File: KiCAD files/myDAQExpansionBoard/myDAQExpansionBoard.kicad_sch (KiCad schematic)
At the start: 48 parts, among them J1 OSTV7XX3151

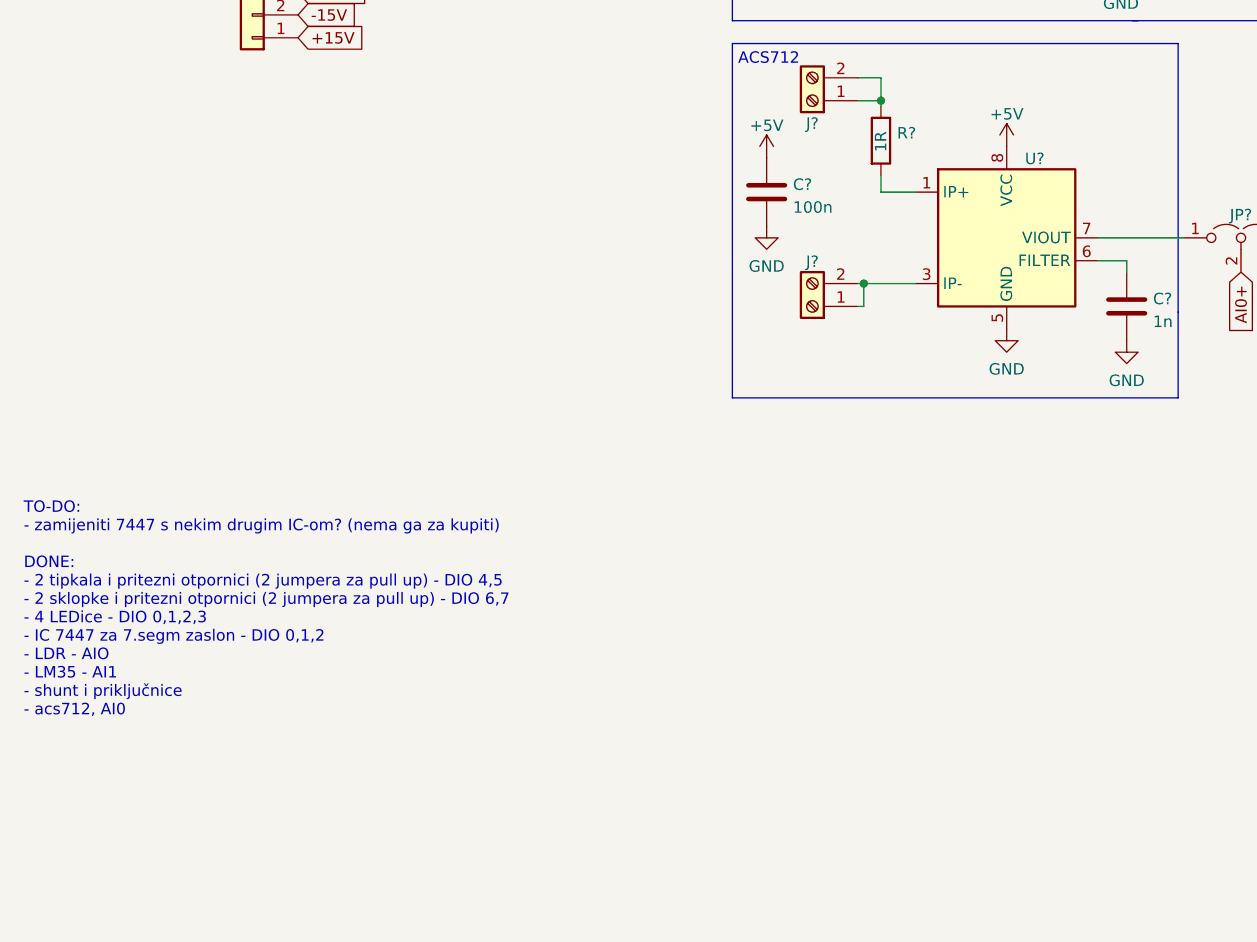
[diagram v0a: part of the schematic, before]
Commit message: update
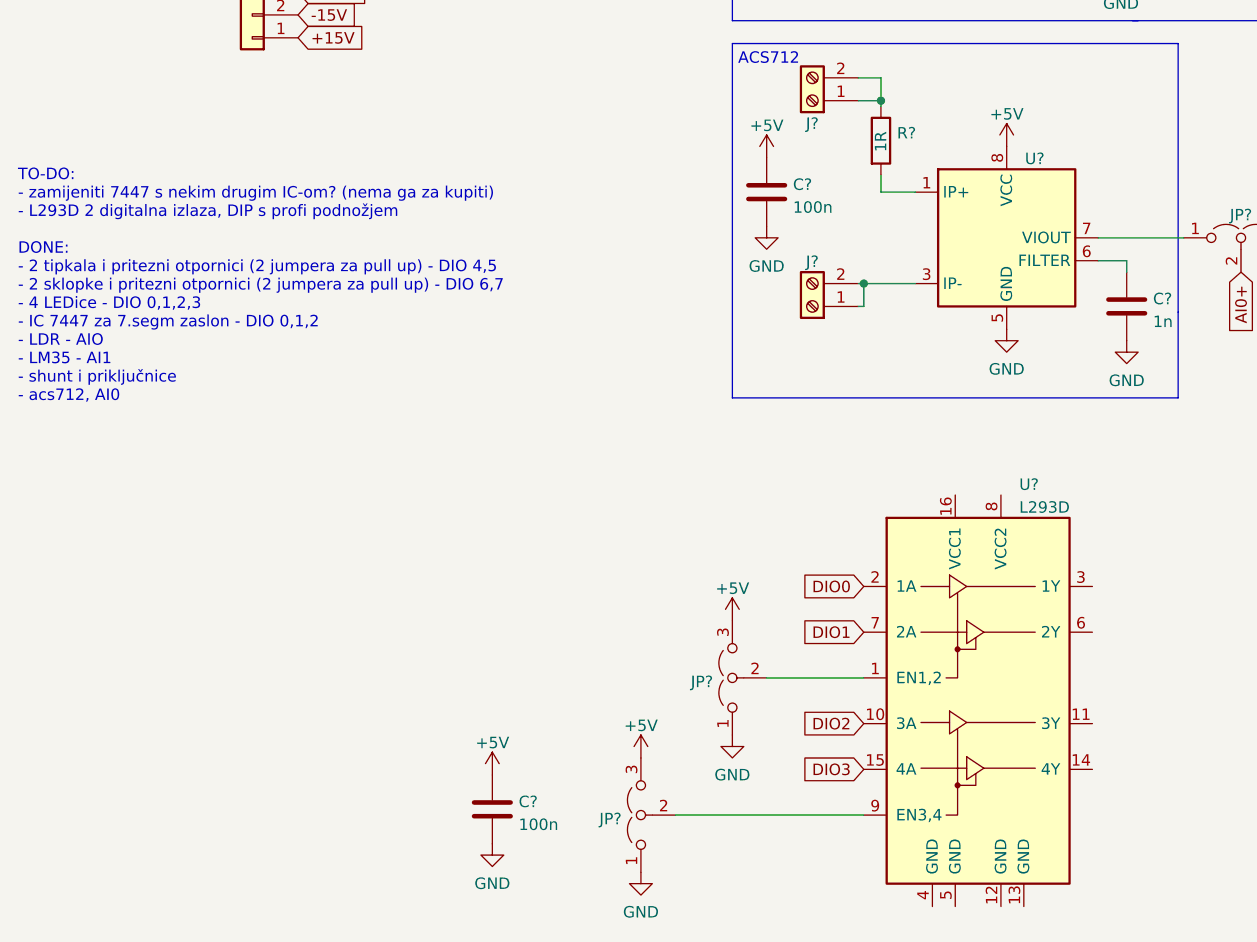
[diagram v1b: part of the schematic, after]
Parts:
- added C?: 100n, symbol Device:C
- added JP? (x2): Jumper_3_Open, symbol Jumper:Jumper_3_Open
- added U?: L293D, Package_DIP:DIP-16_W7.62mm, symbol Driver_Motor:L293D
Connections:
- net +5V: now also C?.1, JP?.3 (B), JP?.3 (B)
- net DIO0: now also U?.2 (1A)
- net DIO1: now also U?.7 (2A)
- net DIO2: now also U?.10 (3A)
- net DIO3: now also U?.15 (4A)
- net GND: now also C?.2, JP?.1 (A), JP?.1 (A)
- new net: JP?.2 (C), U?.1 (EN1,2)
- new net: JP?.2 (C), U?.9 (EN3,4)
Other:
- note added: "TO-DO: - zamijeniti 7447 s nekim drugim IC-om? (nema ga za kupiti) - L293D 2 digitalna izlaza, DIP s profi podnožjem DONE: - 2 tipkala i pritezni otpornici (2 jumpera za pull up) - DIO 4,5 - 2 sklopke i pritezni otpornici (2 jumpera za pull up) - DIO 6,7 - 4 LEDice - DIO 0,1,2,3 - IC 7447 za 7.segm zaslon - DIO 0,1,2 - LDR - AIO - LM35 - AI1 - shunt i priključnice - acs712, AI0"
- note removed: "TO-DO: - zamijeniti 7447 s nekim drugim IC-om? (nema ga za kupiti) DONE: - 2 tipkala i pritezni otpornici (2 jumpera za pull up) - DIO 4,5 - 2 sklopke i pritezni otpornici (2 jumpera za pull up) - DIO 6,7 - 4 LEDice - DIO 0,1,2,3 - IC 7447 za 7.segm zaslon - DIO 0,1,2 - LDR - AIO - LM35 - AI1 - shunt i priključnice - acs712, AI0"

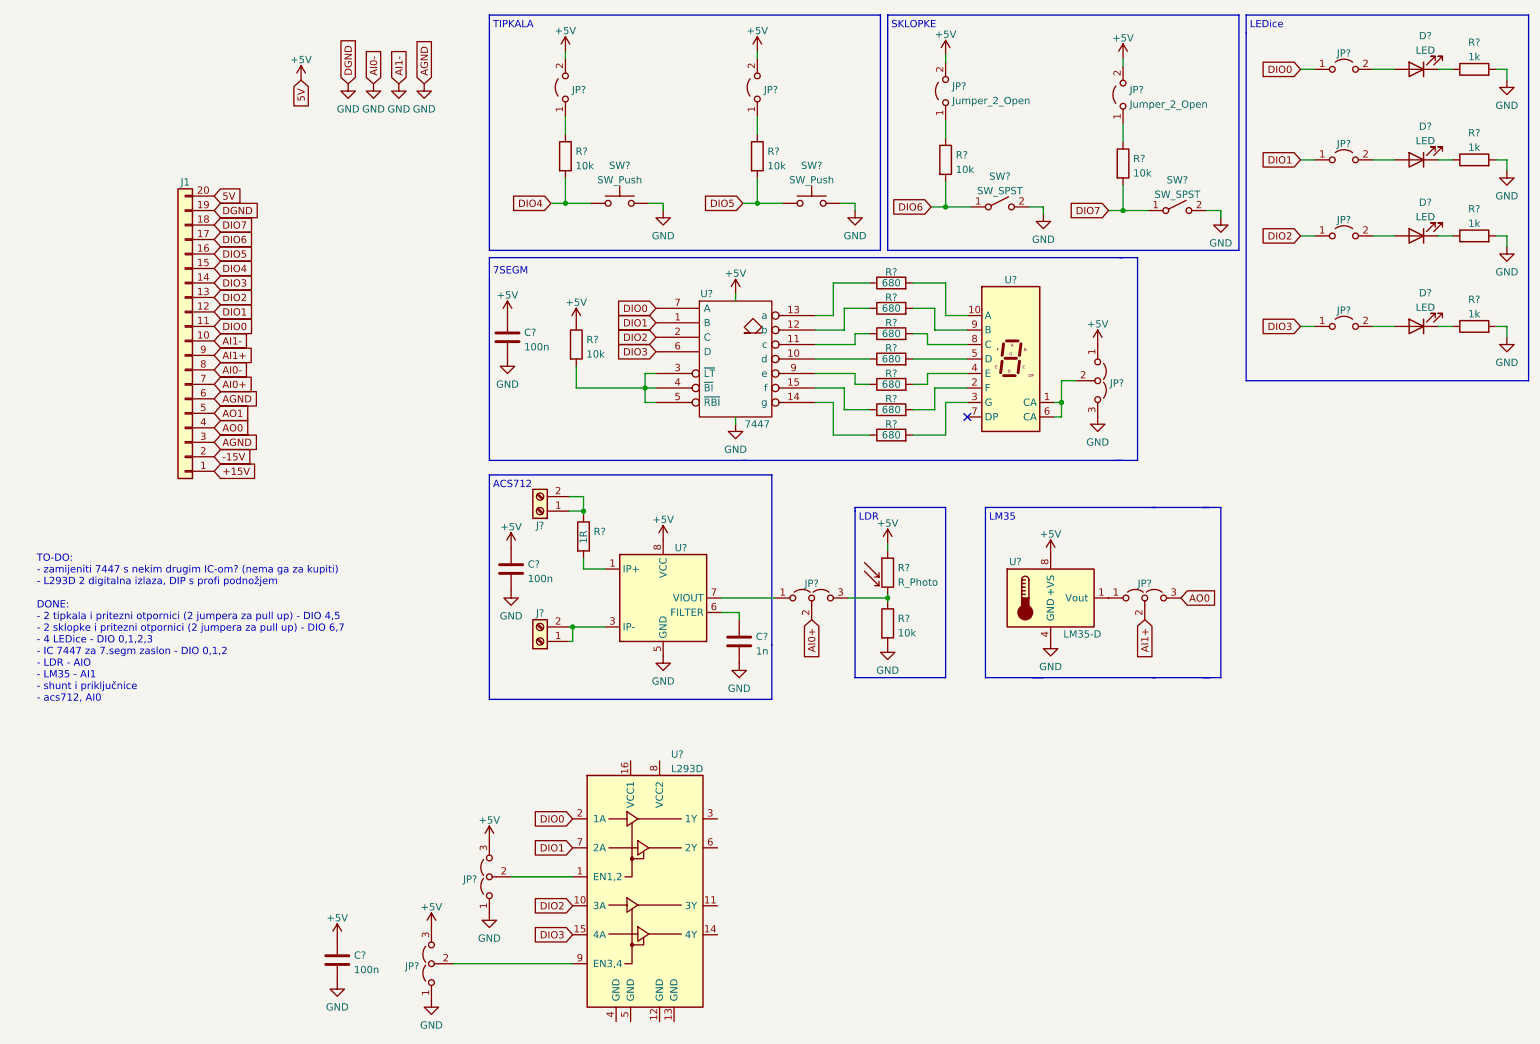
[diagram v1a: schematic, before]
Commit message: Update myDAQExpansionBoard.kicad_sch
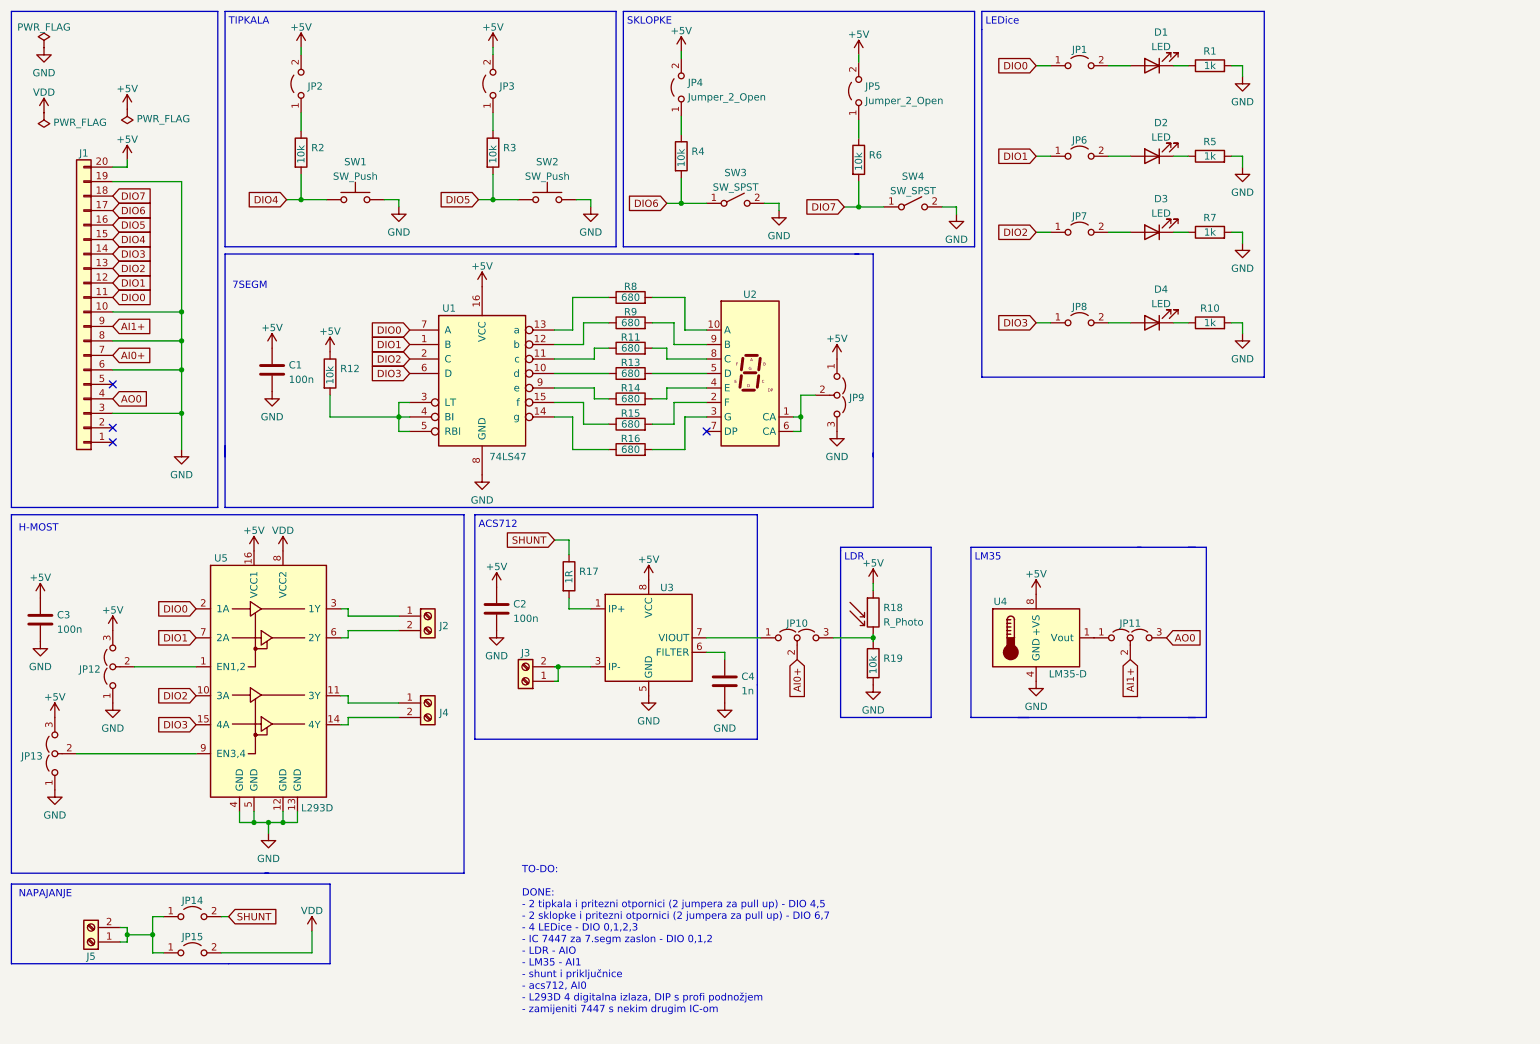
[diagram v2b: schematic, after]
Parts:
- removed U?: 7447, symbol 74xx_IEEE:7447
- added J2, J4: Screw_Terminal_01x02, symbol Connector:Screw_Terminal_01x02
- added JP14, JP15: Jumper_2_Open, symbol Jumper:Jumper_2_Open
- added U1: 74LS47, Package_DIP:DIP-16_W7.62mm, symbol 74xx:74LS47
- D1, D2, D3, D4: renamed from D?; footprint (none) -> LED_THT:LED_D5.0mm
- J1: footprint (none) -> Library:OSTV7XX3151
- gave numbers to parts that had none: 46
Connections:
- net +5V: now also U5.16 (VCC1), U1.16 (VCC)
- net DIO0: now also U1.7 (A)
- net DIO1: now also U1.1 (B)
- net DIO2: now also U1.2 (C)
- net DIO3: now also U1.6 (D)
- net GND: now also U5.12 (GND), U5.13 (GND), U5.4 (GND), U5.5 (GND), U1.8 (GND)
- net at U5.11 (3Y): now also J4.1 (Pin_1)
- net at U5.14 (4Y): now also J4.2 (Pin_2)
- net at U5.3 (1Y): now also J2.1 (Pin_1)
- net at U5.6 (2Y): now also J2.2 (Pin_2)
- net VDD: now reaches U5.8 (VCC2)
- net VDD: now also JP15.2 (B)
- net at R8.1: now also U1.13 (a)
- net at R9.1: now also U1.12 (b)
- net at R13.1: now also U1.10 (d)
- net at R11.1: now also U1.11 (c)
- net at R16.1: now also U1.14 (g)
- net at R15.1: now also U1.15 (f)
- net at R12.2: now also U1.3 (LT), U1.4 (BI), U1.5 (RBI)
- net at R14.1: now also U1.9 (e)
- net at J5.1 (Pin_1), J5.2 (Pin_2): now also JP14.1 (A), JP15.1 (A); no longer R17.1
- net +15V: no longer names the net of J1.1 (Pin_1)
- net -15V: no longer names the net of J1.2 (Pin_2)
- net AO1: no longer names the net of J1.5 (Pin_5)
- new net SHUNT: JP14.2 (B), R17.1
- no-connect marks 1 -> 4
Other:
- note added: "H-MOST"
- note added: "NAPAJANJE"
- note added: "TO-DO: DONE: - 2 tipkala i pritezni otpornici (2 jumpera za pull up) - DIO 4,5 - 2 sklopke i pritezni otpornici (2 jumpera za pull up) - DIO 6,7 - 4 LEDice - DIO 0,1,2,3 - IC 7447 za 7.segm zaslon - DIO 0,1,2 - LDR - AIO - LM35 - AI1 - shunt i priključnice - acs712, AI0 - L293D 4 digitalna izlaza, DIP s profi podnožjem - zamijeniti 7447 s nekim drugim IC-om"
- note removed: "TO-DO: - zamijeniti 7447 s nekim drugim IC-om? (nema ga za kupiti) - L293D 2 digitalna izlaza, DIP s profi podnožjem DONE: - 2 tipkala i pritezni otpornici (2 jumpera za pull up) - DIO 4,5 - 2 sklopke i pritezni otpornici (2 jumpera za pull up) - DIO 6,7 - 4 LEDice - DIO 0,1,2,3 - IC 7447 za 7.segm zaslon - DIO 0,1,2 - LDR - AIO - LM35 - AI1 - shunt i priključnice - acs712, AI0"
- moved on the sheet: C1, C2, C3, C4, D1, D2, D3, D4, J1, J3, J5, JP1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
